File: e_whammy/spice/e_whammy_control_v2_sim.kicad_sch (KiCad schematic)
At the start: 34 parts, among them U1 ${SIM.PARAMS}, U10 OPEN_DRAIN_INVERTER, U2 ${SIM.PARAMS}, U3 OPEN_COLLECTOR_COMPARATOR, U4 OPEN_COLLECTOR_COMPARATOR, U5 ADG779, U6 ADG779, U7 OPEN_DRAIN_INVERTER, U9 OPEN_DRAIN_INVERTER

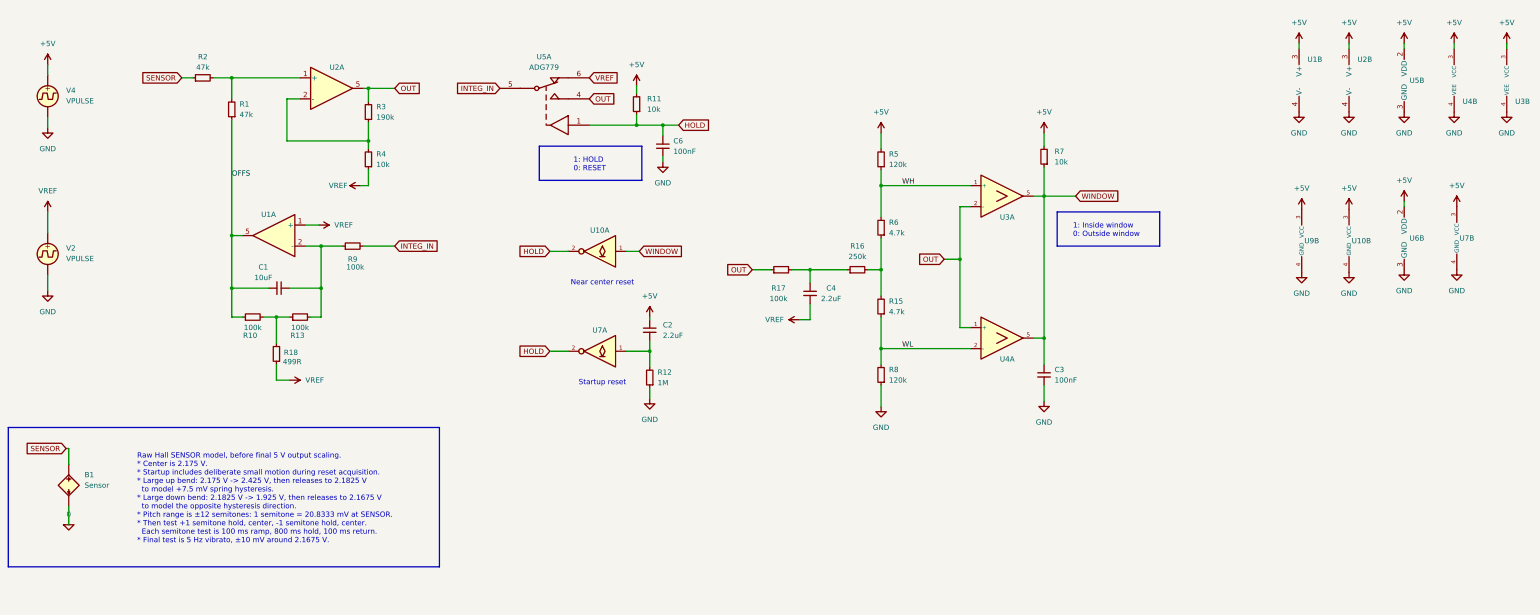
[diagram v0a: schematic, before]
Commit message: - Cleanup - Simplification
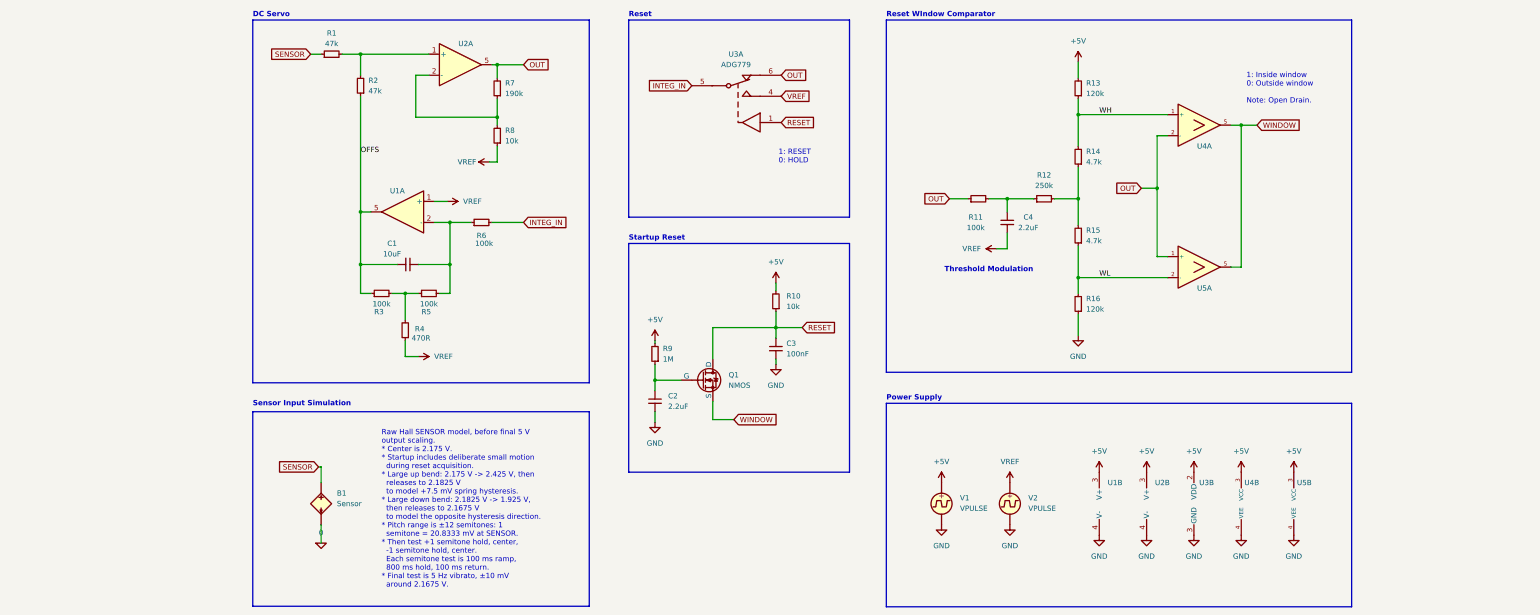
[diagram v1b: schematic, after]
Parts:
- removed C3: 100nF, symbol Device:C_Small
- removed R7: 10k, symbol Device:R_Small
- removed U10, U7, U9: OPEN_DRAIN_INVERTER, symbol cycfi_spice_library:OPEN_DRAIN_INVERTER
- removed U6: ADG779, KS_6_ADI, symbol cycfi_spice_library:ADG779
- added Q1: NMOS, symbol Simulation_SPICE:NMOS
- R4: renamed from R18; value 499R -> 470R
- renumbered C6 to C3, R2 to R1, R11 to R10, R17 to R11, R16 to R12, R5 to R13, R6 to R14, R8 to R16, R1 to R2, R10 to R3, R13 to R5, R9 to R6, R3 to R7, R4 to R8, R12 to R9, U5 to U3, U3 to U4, U3 to U5, U4 to U5, V4 to V1
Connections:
- net +5V: now also R9.2; no longer C2.1
- net GND: now also C2.2; no longer R9.1
- net OUT: now also U3.6; no longer U3.4
- net VREF: now also U3.4; no longer U3.6
- net WINDOW: now also Q1.3 (S)
- net HOLD renamed RESET
- net RESET: now also Q1.1 (D)
- new net: C2.1, Q1.2 (G), R9.1
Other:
- note added: "1: Inside window 0: Outside window Note: Open Drain."
- note added: "1: RESET 0: HOLD"
- note added: "DC Servo"
- note added: "Power Supply"
- note added: "Reset"
- note added: "Reset WIndow Comparator"
- note added: "Sensor Input Simulation"
- note added: "Startup Reset"
- note added: "Threshold Modulation"
- note removed: "1: HOLD 0: RESET"
- note removed: "1: Inside window 0: Outside window"
- note removed: "Near center reset"
- note removed: "Startup reset"
- moved on the sheet: B1, C1, C2, C3, C4, R1, R10, R11, R12, R13, R14, R15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
